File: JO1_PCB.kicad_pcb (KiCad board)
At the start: 2 copper layers, 60 x 90 mm, 19 parts, among them J1 CN8, J10 ESC_PWM, J11 CAN_WCMCU-1051_BLUEPILL, J2 CN7, J3 CN9, J4 CN10, J5 MPU-6050, J6 CAN_WCMCU-1051_NUCLEO, J7 SERVO, J8 DC_MOTOR, J9 ESC_MOTOR, U1 NRF24L01, U2 BP

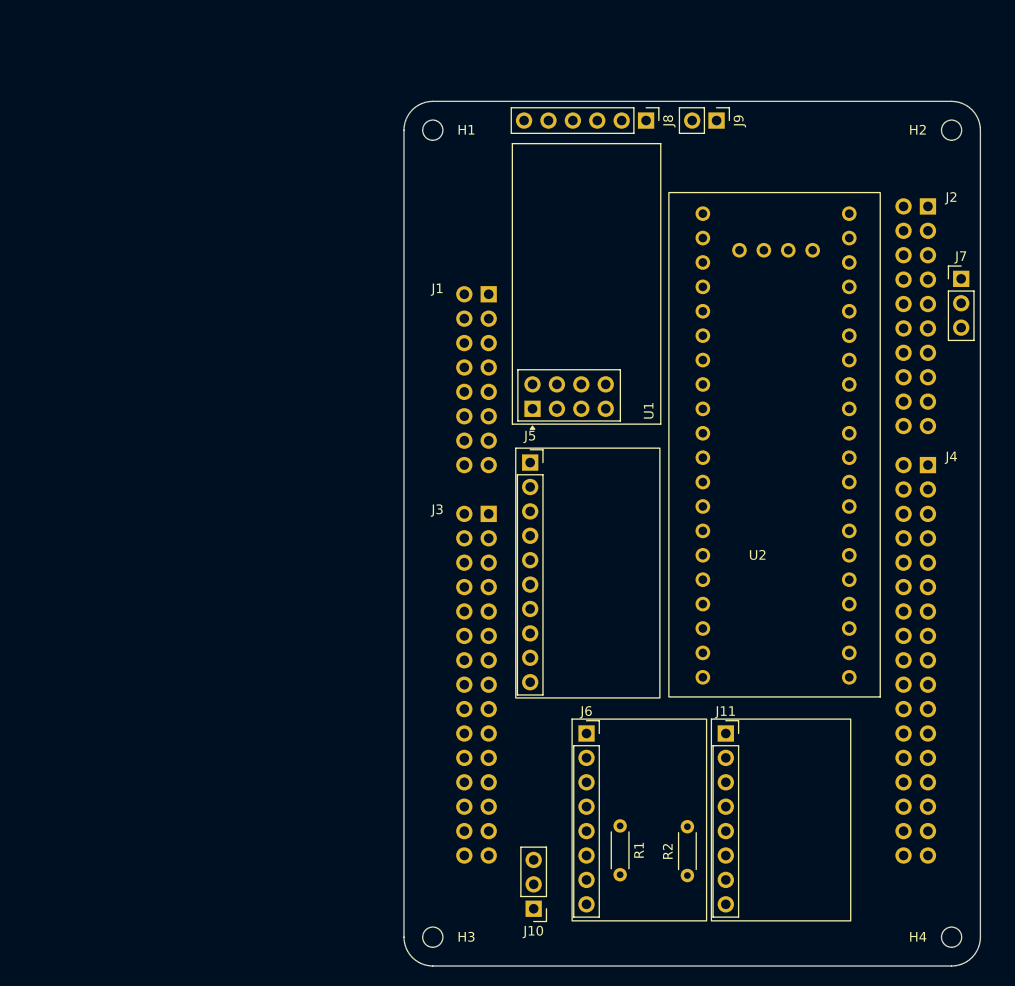
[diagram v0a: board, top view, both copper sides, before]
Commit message: Routing
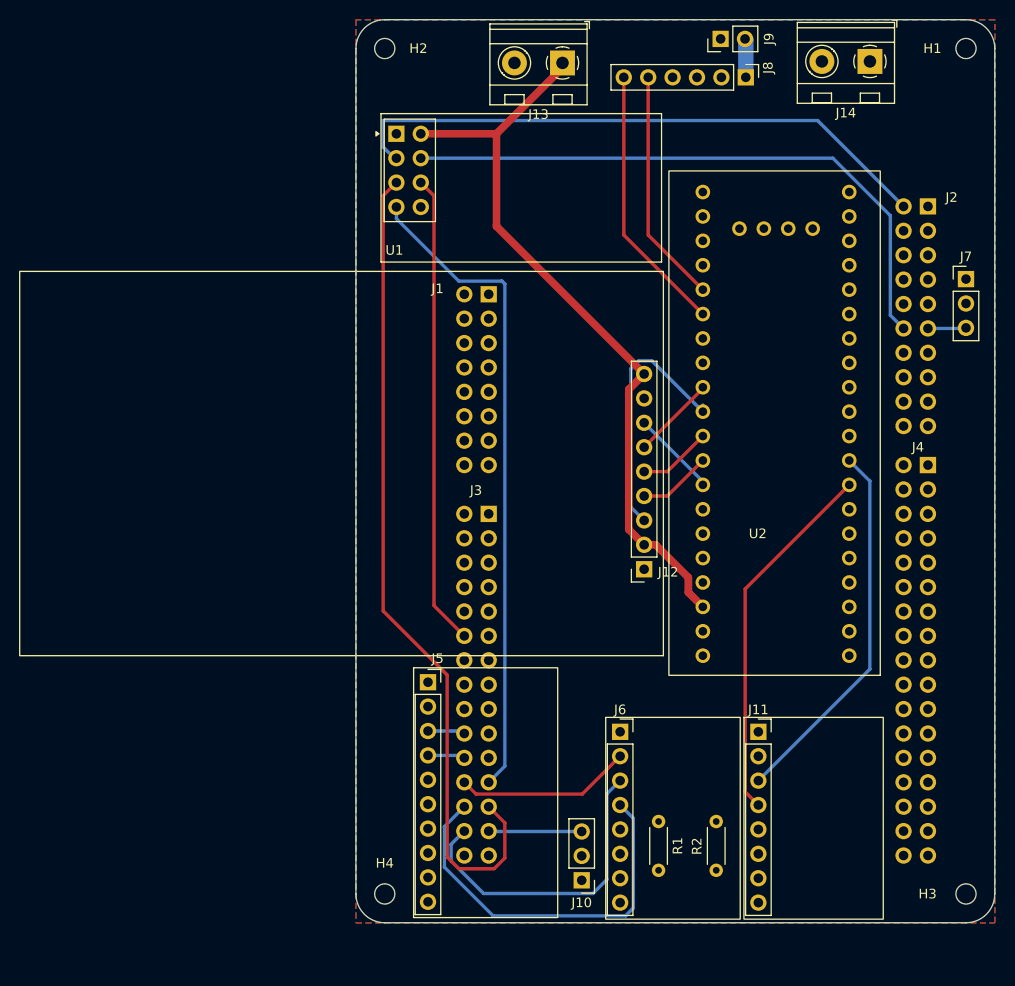
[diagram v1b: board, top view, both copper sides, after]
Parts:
- added J12: TFT, Connector_PinSocket_2.54mm:PinSocket_1x09_P2.54mm_Vertical, F.Cu at (125.5, 100.7)
- added J13: LM2596_3.3V, TerminalBlock_MetzConnect:TerminalBlock_MetzConnect_Type094_RT03502HBLU_1x02_P5.00mm_Horizontal, F.Cu at (117.0, 48.0)
- added J14: LM2596_5V, TerminalBlock_MetzConnect:TerminalBlock_MetzConnect_Type094_RT03502HBLU_1x02_P5.00mm_Horizontal, F.Cu at (149.0, 47.8)
- moved H2 59.6 mm to (98.5, 46.5)
- moved H4 59.2 mm to (98.5, 134.5)
- moved H1 56.1 mm to (159.0, 46.5)
- moved H3 55.7 mm to (159.0, 134.5)
- moved U1 31.9 mm to (99.7, 55.4), turned to 0 degrees
- moved J5 25.2 mm to (103.0, 112.5)
- moved J8 11.3 mm to (136.1, 49.5)
- moved J9 8.51 mm to (133.5, 45.5), turned to 90 degrees
- moved J10 5.81 mm to (119.0, 133.1)
- moved R1 4.03 mm to (127.0, 132.0)
- moved J6 3.50 mm to (123.0, 117.6)
- moved J11 3.39 mm to (137.4, 117.6)
- moved R2 3.05 mm to (133.0, 132.0)
- moved U2 2.25 mm to (137.3, 88.7)
- moved J7 0.50 mm to (159.0, 70.5)
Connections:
- J1 pad GND: unconnected-(J1-11-PadGND) -> GND
- J2 pad GND: unconnected-(J2-8-PadGND) -> GND
- J3 pad GND: unconnected-(J3-12-PadGND) -> GND
- J4 pad GND: unconnected-(J4-5-PadGND) -> GND
- U2 pad 3V3: unconnected-(U2-3.3V-Pad3V3) -> 3.3V
- U2 pad G: unconnected-(U2-GND-PadG) -> GND
- U2 pad PA0: unconnected-(U2-PadPA0) -> BLUEPILL_ENCODER_A
- U2 pad PA1: unconnected-(U2-PadPA1) -> BLUEPILL_ENCODER_B
- U2 pad PA4: unconnected-(U2-PadPA4) -> BLUEPILL_TFT_RESET
- U2 pad PA5: unconnected-(U2-PadPA5) -> BLUEPILL_TFT_CLK
- U2 pad PA6: unconnected-(U2-PadPA6) -> BLUEPILL_TFT_DC
- U2 pad PA7: unconnected-(U2-PadPA7) -> BLUEPILL_TFT_MOSI
- U2 pad PB0: unconnected-(U2-PadPB0) -> BLUEPILL_TFT_CS
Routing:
- net NUCLEO_NRF_SPI5_SCK: track 0.00 -> 86.5 mm
- net 3.3V: track 0.00 -> 77.8 mm
- net NUCLEO_NRF_SPI5_MISO: track 0.00 -> 67.9 mm
- net NUCLEO_NRF_CSN: track 0.00 -> 63.7 mm
- net NUCLEO_NRF_CE: track 0.00 -> 62.5 mm
- net NUCLEO_NRF_SPI5_MOSI: track 0.00 -> 49.1 mm
- net NUCLEO_FDCAN_RX: track 0.00 -> 40.5 mm
- net BLUEPILL_CAN_TX: track 0.00 -> 39.0 mm
- net BLUEPILL_CAN_RX: track 0.00 -> 38.4 mm
- net NUCLEO_FDCAN_TX: track 0.00 -> 32.8 mm
- net BLUEPILL_ENCODER_B: track 0.00 -> 28.0 mm
- net BLUEPILL_TFT_CLK: track 0.00 -> 27.1 mm
- net BLUEPILL_ENCODER_A: track 0.00 -> 24.5 mm
- net GND: track 0.00 -> 18.4 mm
- net NUCLEO_ESC_TIM14_CH1: track 0.00 -> 10.3 mm
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- added copper zone on B.Cu, net 5V
- added copper zone on F.Cu, net GND
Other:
- board size 60 x 90 mm -> 66.5 x 94 mm
